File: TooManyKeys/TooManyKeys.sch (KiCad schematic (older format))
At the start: 60 parts, among them J1 54104-3031_Oled, J2 AVR-ISP-6(SWR204-NRTN-D03-RA-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, SW1 SW_Push, U1 PRTR5V0U2X, U2 AT90USB1286-AU, U3 PCA9306, U4 AZ1117CH-3.3TRG1, Y1 16MHz

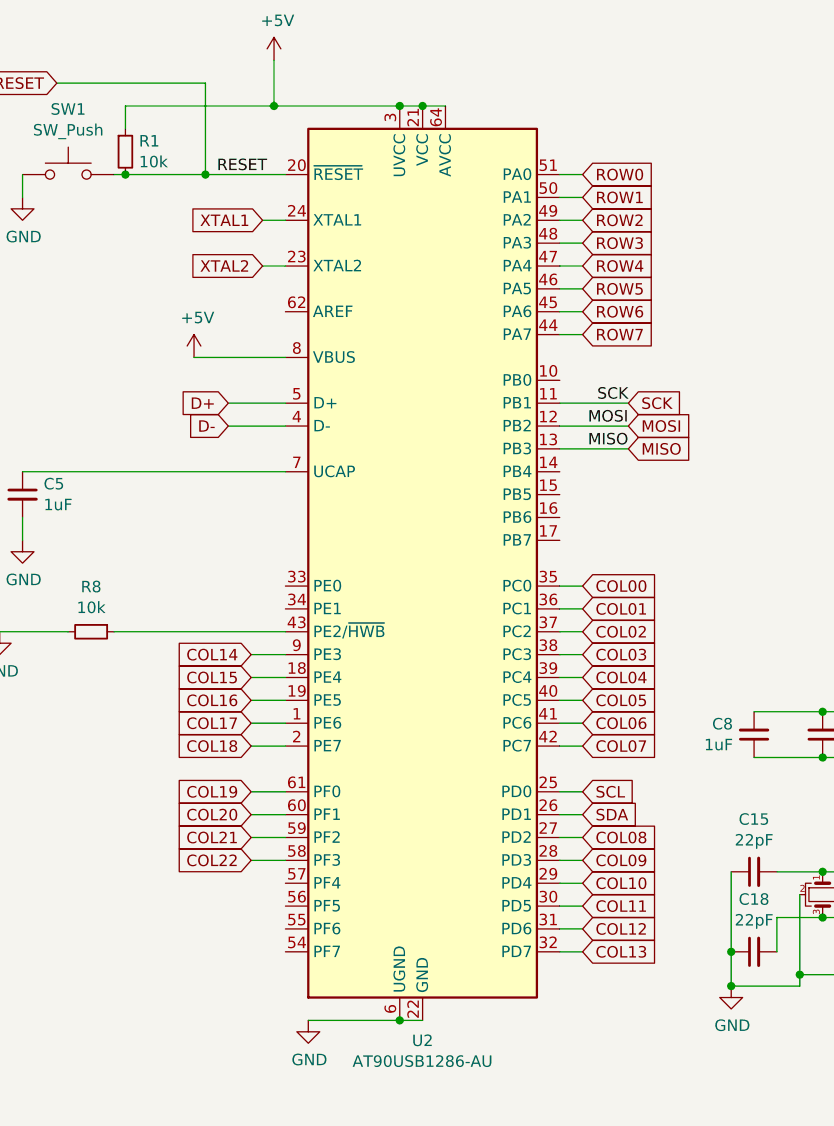
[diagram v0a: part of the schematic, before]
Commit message: New footprint, pcb key matrix completed
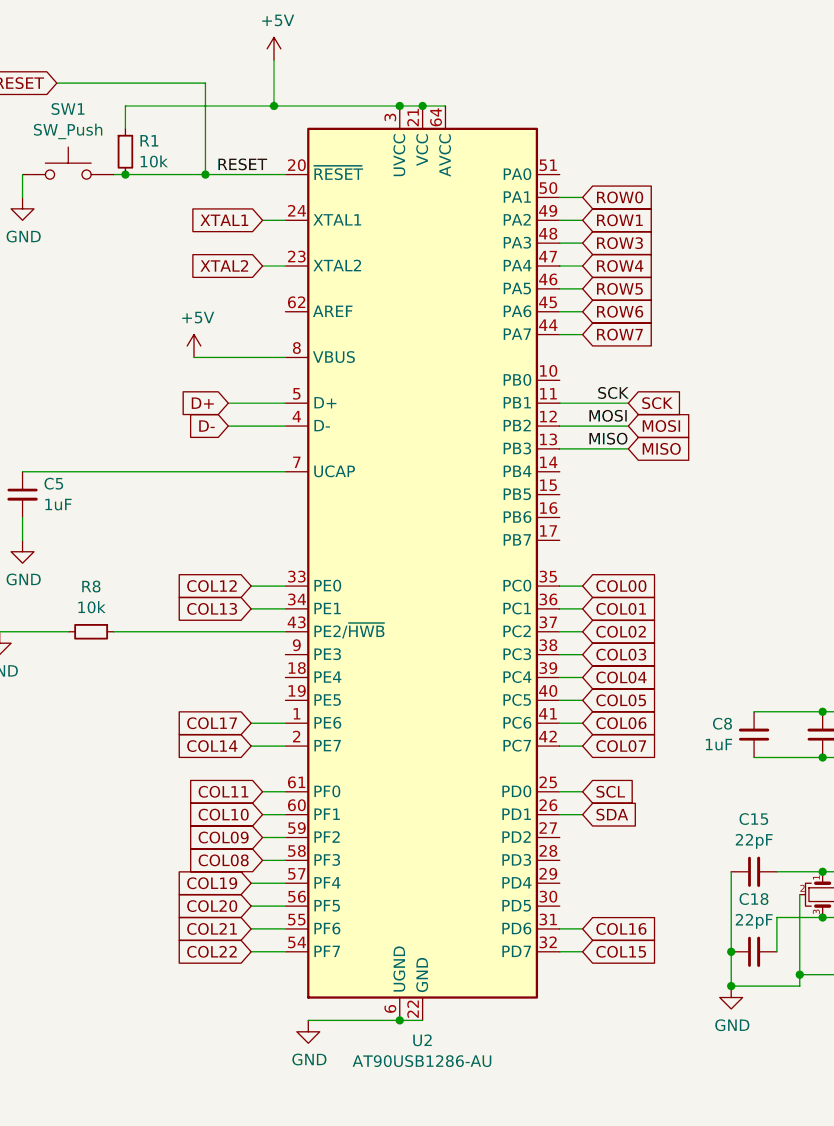
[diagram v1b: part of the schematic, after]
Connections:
- net COL18 is gone; now on net COL14: U2.2 (PE7)
- net ROW2 is gone; now on net ROW1: U2.49 (PA2)
- net COL08: now also U2.58 (PF3); no longer U2.27 (PD2)
- net COL09: now also U2.59 (PF2); no longer U2.28 (PD3)
- net COL10: now also U2.60 (PF1); no longer U2.29 (PD4)
- net COL11: now also U2.61 (PF0); no longer U2.30 (PD5)
- net COL12: now also U2.33 (PE0); no longer U2.31 (PD6)
- net COL13: now also U2.34 (PE1); no longer U2.32 (PD7)
- net COL14: no longer U2.9 (PE3)
- net COL15: now also U2.32 (PD7); no longer U2.18 (PE4)
- net COL16: now also U2.31 (PD6); no longer U2.19 (PE5)
- net COL19: now also U2.57 (PF4); no longer U2.61 (PF0)
- net COL20: now also U2.56 (PF5); no longer U2.60 (PF1)
- net COL21: now also U2.55 (PF6); no longer U2.59 (PF2)
- net COL22: now also U2.54 (PF7); no longer U2.58 (PF3)
- net ROW0: now also U2.50 (PA1); no longer U2.51 (PA0)
- net ROW1: no longer U2.50 (PA1)
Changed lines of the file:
@@
 Text GLabel 9050 1500 2    50   Input ~ 0
 D-
-$Sheet
-S 1850 6650 1100 550
-U 5E8A6E89
-F0 "Matrix" 50
-F1 "Matrix.sch" 50
-$EndSheet
 $Comp
 L TooManyKeys-rescue:HRO-TYPE-C-31-M-12-Type-C USB1
@@
 Text GLabel 3700 4000 2    50   Input ~ 0
 SDA
-Text GLabel 3700 1300 2    50   Input ~ 0
+Text GLabel 3700 1400 2    50   Input ~ 0
 ROW1
-Text GLabel 3700 1400 2    50   Input ~ 0
-ROW2
 Text GLabel 3700 1500 2    50   Input ~ 0
 ROW3
@@
 Text GLabel 3700 1900 2    50   Input ~ 0
 ROW7
-Text GLabel 3700 1200 2    50   Input ~ 0
+Text GLabel 3700 1300 2    50   Input ~ 0
 ROW0
 Text GLabel 3700 3000 2    50   Input ~ 0
@@
 Text GLabel 3700 3700 2    50   Input ~ 0
 COL07
-Text GLabel 3700 4100 2    50   Input ~ 0
+Text GLabel 2300 4200 0    50   Input ~ 0
 COL08
-Text GLabel 3700 4200 2    50   Input ~ 0
+Text GLabel 2300 4100 0    50   Input ~ 0
 COL09
-Text GLabel 3700 4300 2    50   Input ~ 0
+Text GLabel 2300 4000 0    50   Input ~ 0
 COL10
-Text GLabel 3700 4400 2    50   Input ~ 0
+Text GLabel 2300 3900 0    50   Input ~ 0
 COL11
+Text GLabel 2250 3000 0    50   Input ~ 0
+COL12
+Text GLabel 2250 3100 0    50   Input ~ 0
+COL13
+Text GLabel 2250 3700 0    50   Input ~ 0
+COL14
+Text GLabel 3700 4600 2    50   Input ~ 0
+COL15
 Text GLabel 3700 4500 2    50   Input ~ 0
-COL12
-Text GLabel 3700 4600 2    50   Input ~ 0
-COL13
-Text GLabel 2250 3300 0    50   Input ~ 0
-COL14
-Text GLabel 2250 3400 0    50   Input ~ 0
-COL15
-Text GLabel 2250 3500 0    50   Input ~ 0
 COL16
 Text GLabel 2250 3600 0    50   Input ~ 0
 COL17
-Text GLabel 2250 3700 0    50   Input ~ 0
-COL18
-Text GLabel 2250 3900 0    50   Input ~ 0
+Text GLabel 2250 4300 0    50   Input ~ 0
 COL19
-Text GLabel 2250 4000 0    50   Input ~ 0
+Text GLabel 2250 4400 0    50   Input ~ 0
 COL20
-Text GLabel 2250 4100 0    50   Input ~ 0
+Text GLabel 2250 4500 0    50   Input ~ 0
 COL21
-Text GLabel 2250 4200 0    50   Input ~ 0
+Text GLabel 2250 4600 0    50   Input ~ 0
 COL22
-$Sheet
-S 3050 6650 1000 550
-U 6065500F
-F0 "Led" 50
-F1 "Led.sch" 50
-$EndSheet
 Wire Wire Line
 	10800 1750 12050 1750
@@
 Text GLabel 15550 6400 2    50   Input ~ 0
 CS28
-$Comp
-L TooManyKeys-rescue:505110-3091_Oled-SamacSys_Parts J1
-U 1 1 604722A8
-P 13050 1050
-F 0 "J1" H 13550 1315 50  0000 C CNN
-F 1 "54104-3031_Oled" H 13550 1224 50  0000 C CNN
-F 2 "SamacSys_Parts:0541043033" H 13900 1150 50  0001 L CNN
-F 3 "https://componentsearchengine.com/Datasheets/1/505110-3091.pdf" H 13900 1050 50  0001 L CNN
-F 4 "MOLEX - 505110-3091 - CONNECTOR, FFC/FPC, 30POS, 1ROW, 0.5MM" H 13900 950 50  0001 L CNN "Description"
-F 5 "2.1" H 13900 850 50  0001 L CNN "Height"
-F 6 "538-505110-3091" H 13900 750 50  0001 L CNN "Mouser Part Number"
-F 7 "https://www.mouser.com/Search/Refine.aspx?Keyword=538-505110-3091" H 13900 650 50  0001 L CNN "Mouser Price/Stock"
-F 8 "Molex" H 13900 550 50  0001 L CNN "Manufacturer_Name"
-F 9 "505110-3091" H 13900 450 50  0001 L CNN "Manufacturer_Part_Number"
-	1    13050 1050
-	-1   0    0    -1
-$EndComp
 Text GLabel 11300 6850 2    50   Input ~ 0
 CS1
@@
 	3600 4000 3700 4000
 Wire Wire Line
-	3700 4100 3600 4100
-Wire Wire Line
-	3700 4200 3600 4200
-Wire Wire Line
-	3700 4300 3600 4300
-Wire Wire Line
-	3700 4400 3600 4400
+	2300 4200 2400 4200
+Wire Wire Line
+	2300 4100 2400 4100
+Wire Wire Line
+	2300 4000 2400 4000
+Wire Wire Line
+	2300 3900 2400 3900
 Wire Wire Line
 	3600 4500 3700 4500
@@
 	3700 4600 3600 4600
 Wire Wire Line
-	2250 3300 2400 3300
-Wire Wire Line
-	2250 3400 2400 3400
-Wire Wire Line
-	2250 3500 2400 3500
+	2250 3700 2400 3700
+Wire Wire Line
+	2250 3000 2400 3000
+Wire Wire Line
+	2250 3100 2400 3100
 Wire Wire Line
 	2250 3600 2400 3600
 Wire Wire Line
-	2250 3700 2400 3700
-Wire Wire Line
-	2250 3900 2400 3900
-Wire Wire Line
-	2250 4000 2400 4000
-Wire Wire Line
-	2250 4100 2400 4100
-Wire Wire Line
-	2250 4200 2400 4200
+	2250 4300 2400 4300
+Wire Wire Line
+	2250 4400 2400 4400
+Wire Wire Line
+	2250 4500 2400 4500
+Wire Wire Line
+	2250 4600 2400 4600
 Wire Wire Line
 	2400 2200 2150 2200
@@
 Text Label 3900 2200 2    50   ~ 0
 SCK
-Wire Wire Line
-	3700 1200 3600 1200
 Wire Wire Line
 	3700 1300 3600 1300
@@
 	1700 1200 2050 1200
 Connection ~ 2050 1200
+$Comp
+L TooManyKeys-rescue:505110-3091_Oled-SamacSys_Parts J1
+U 1 1 604722A8
+P 13050 1050
+F 0 "J1" H 13550 1315 50  0000 C CNN
+F 1 "54104-3031_Oled" H 13550 1224 50  0000 C CNN
+F 2 "SamacSys_Parts:0541043033" H 13900 1150 50  0001 L CNN
+F 3 "https://componentsearchengine.com/Datasheets/1/505110-3091.pdf" H 13900 1050 50  0001 L CNN
+F 4 "MOLEX - 505110-3091 - CONNECTOR, FFC/FPC, 30POS, 1ROW, 0.5MM" H 13900 950 50  0001 L CNN "Description"
+F 5 "2.1" H 13900 850 50  0001 L CNN "Height"
+F 6 "538-505110-3091" H 13900 750 50  0001 L CNN "Mouser Part Number"
+F 7 "https://www.mouser.com/Search/Refine.aspx?Keyword=538-505110-3091" H 13900 650 50  0001 L CNN "Mouser Price/Stock"
+F 8 "Molex" H 13900 550 50  0001 L CNN "Manufacturer_Name"
+F 9 "505110-3091" H 13900 450 50  0001 L CNN "Manufacturer_Part_Number"
+	1    13050 1050
+	-1   0    0    -1
+$EndComp
+$Sheet
+S 3050 6650 1000 550
+U 6065500F
+F0 "Led" 50
+F1 "Led.sch" 50
+$EndSheet
+$Sheet
+S 1850 6650 1100 550
+U 5E8A6E89
+F0 "Matrix" 50
+F1 "Matrix.sch" 50
+$EndSheet
 $EndSCHEMATC
